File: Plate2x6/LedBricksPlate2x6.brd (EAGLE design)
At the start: 44 x 12 mm, 8 parts, among them J1 SM02B-SRSS-TB, J2 SM02B-SRSS-TB

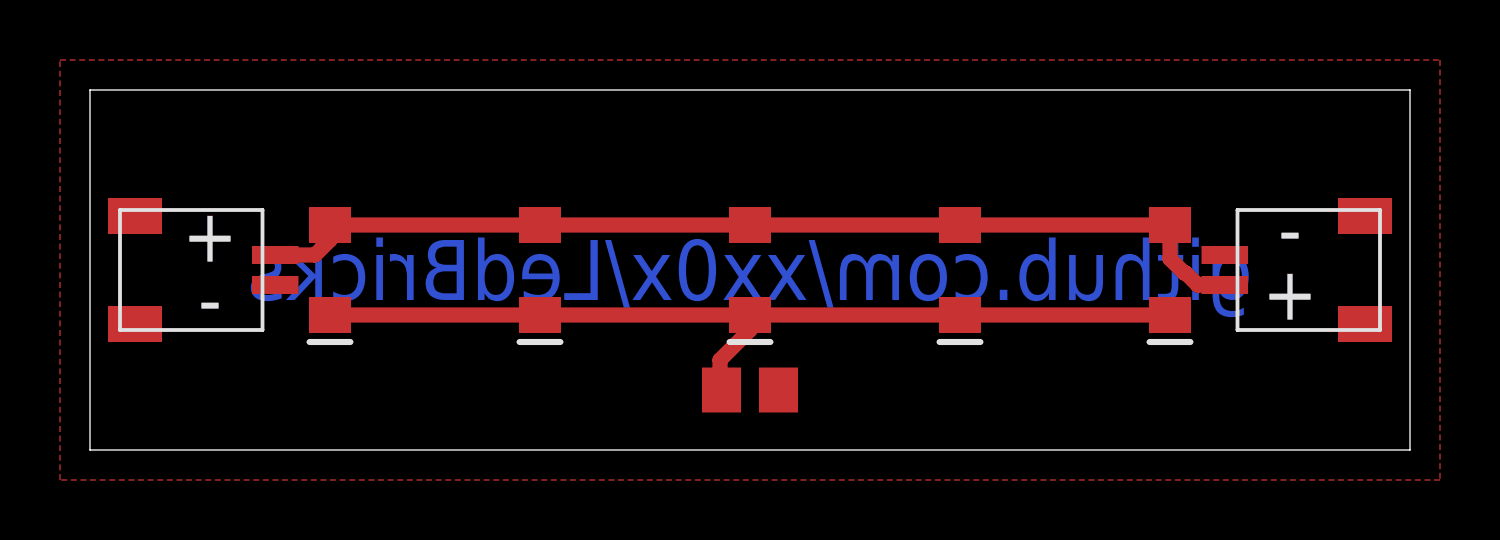
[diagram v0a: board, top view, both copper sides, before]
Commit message: gerbers, pnp file
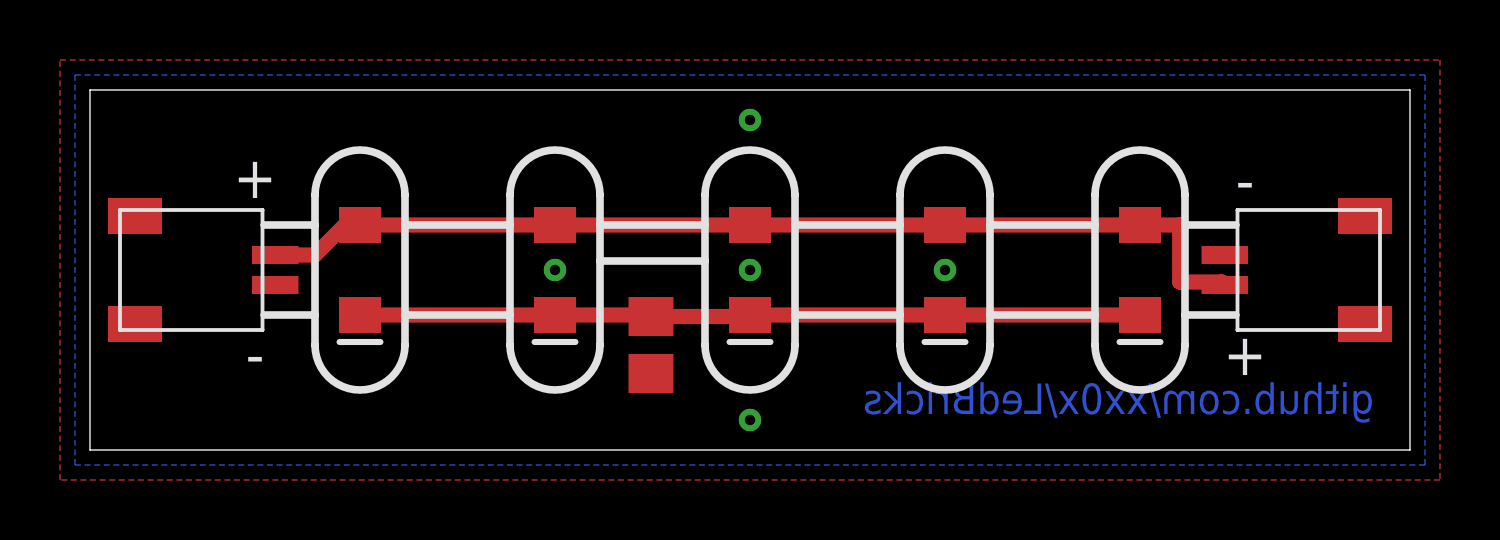
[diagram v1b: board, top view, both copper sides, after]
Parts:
- D1, D2, D3, D4, D5: value (none) -> XL-3216WWC
- moved R1 3.62 mm to (18.7, 3.50), turned to 90 degrees
- moved D1 1.00 mm to (9.00, 6.00)
- moved D5 1.00 mm to (35.0, 6.00)
- moved D2 0.50 mm to (15.5, 6.00)
- moved D4 0.50 mm to (28.5, 6.00)
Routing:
- net N$2: track 30.9 -> 26.0 mm
- added copper zone on layer 16, net GND
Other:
- board text added: "+"
- board text added: "-"
- board text removed: "+ -"
- board text removed: "- +"
